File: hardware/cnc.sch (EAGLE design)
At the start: 48 parts, among them IC1 STM32F10XVXT6, Q1 8M, Q2 32K, SW1 SWITCH-SWT-9, SW10 SWITCH-SWT-9, SW11 SWITCH-SWT-9, SW12 SWITCH-SWT-9, SW13 SWITCH-SWT-9, SW14 SWITCH-SWT-9, SW15 SWITCH-SWT-9, SW16 SWITCH-SWT-9, SW2 SWITCH-SWT-9, SW3 SWITCH-SWT-9, SW4 SWITCH-SWT-9, SW5 SWITCH-SWT-9, SW6 SWITCH-SWT-9, SW7 SWITCH-SWT-9, SW8 SWITCH-SWT-9, SW9 SWITCH-SWT-9, U1 LMR14206

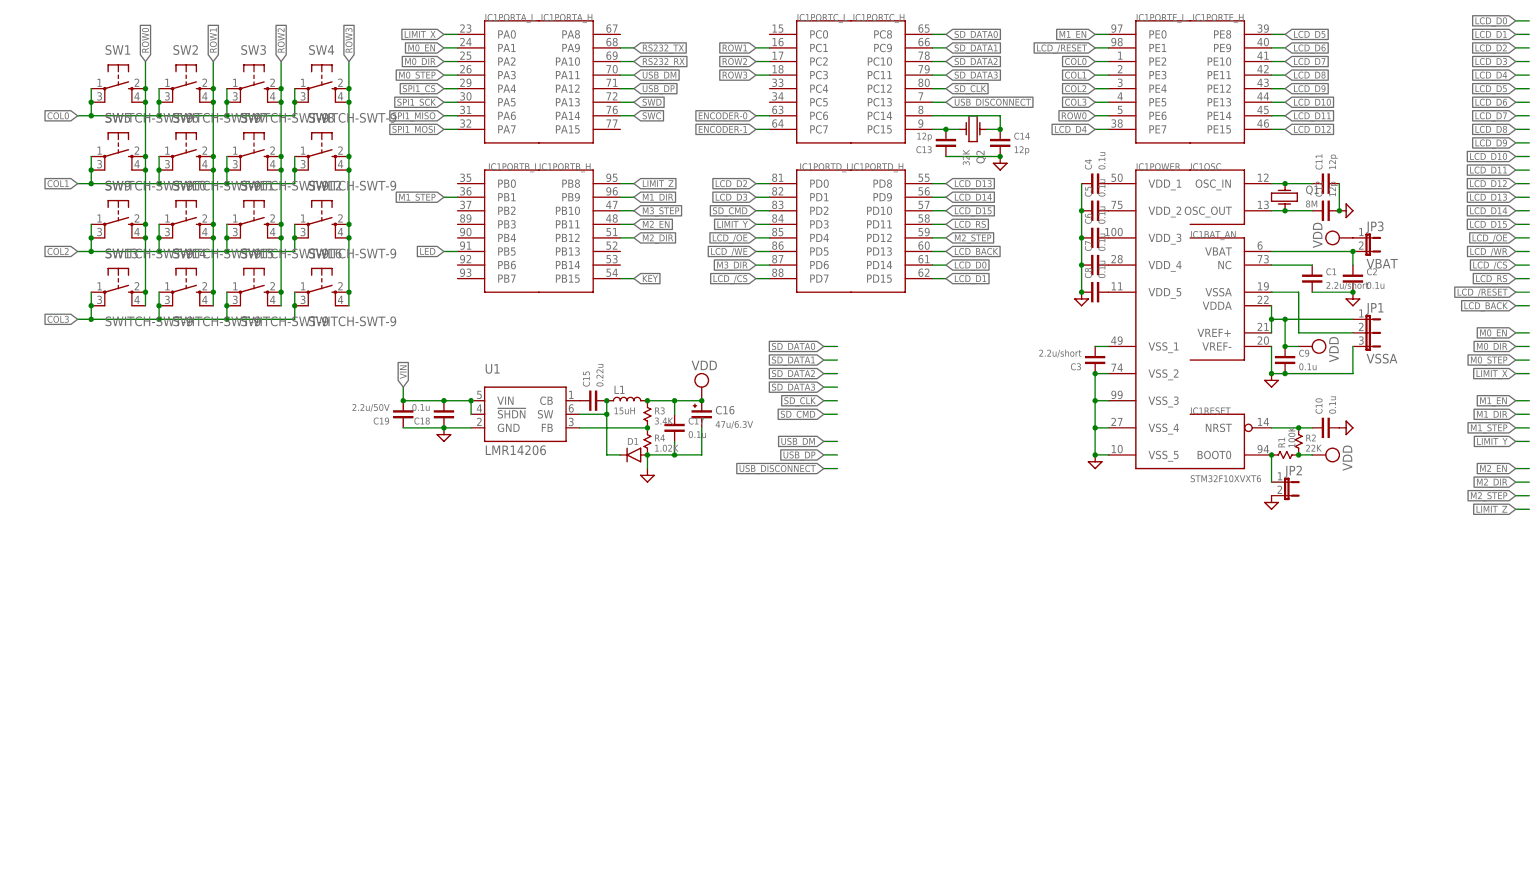
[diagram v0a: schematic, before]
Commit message: Minor changes
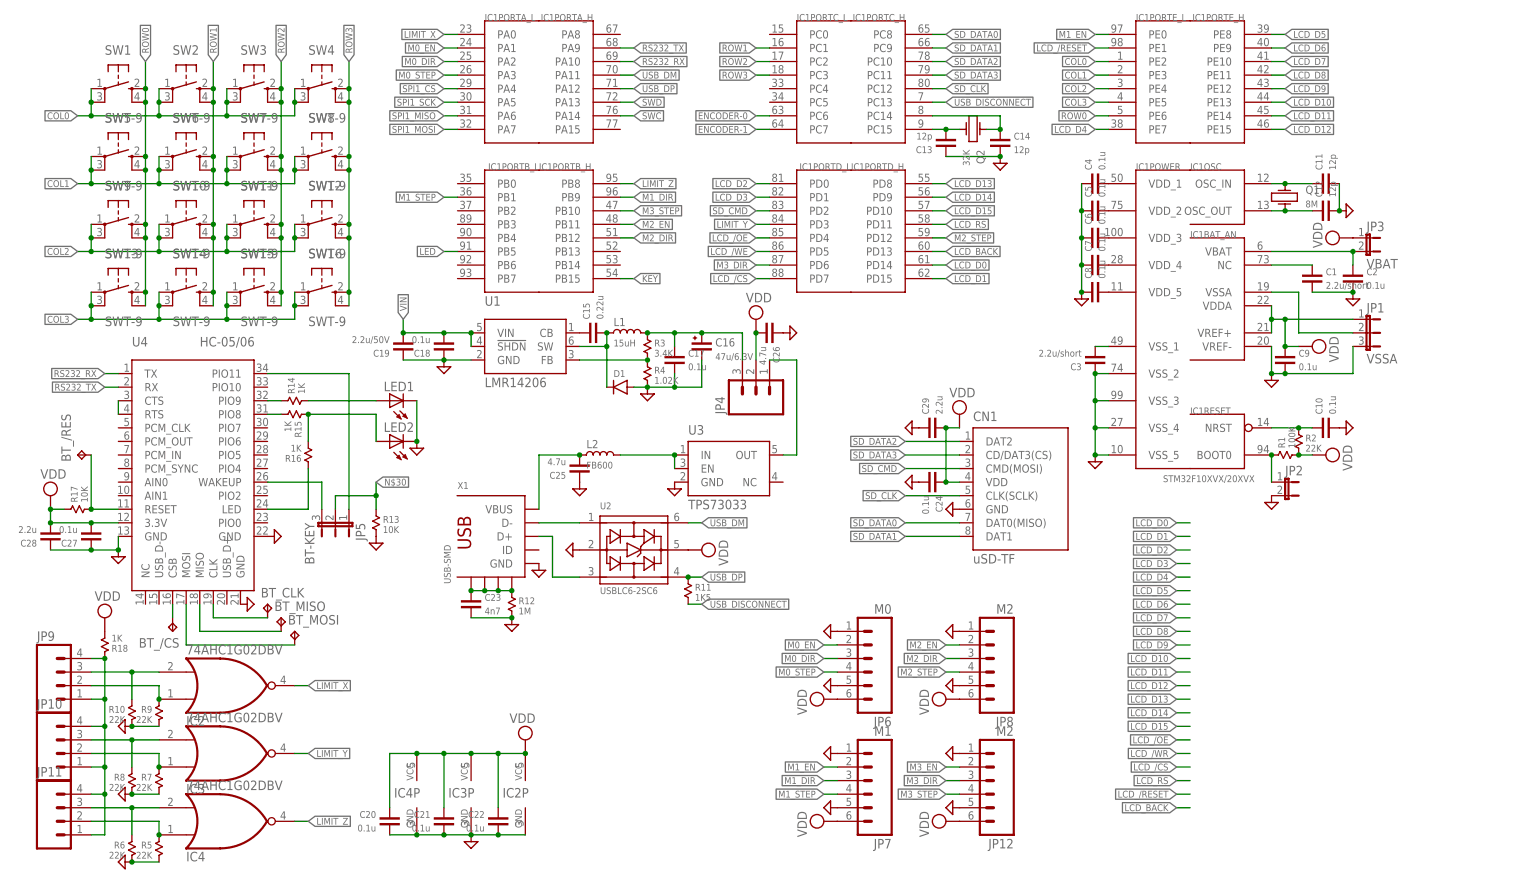
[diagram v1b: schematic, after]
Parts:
- added BT_/CS, BT_/RES, BT_CLK, BT_MISO, BT_MOSI: TPTP12R, testpad:TPTP12R
- added C20, C21, C22, C24, C27: 0.1u, X893:CAP-0603
- added C23: 4n7, X893:CAP-0603
- added C25, C26: 4.7u, X893:CAP-0603
- added C28, C29: 2.2u, X893:CAP-0603
- added CN1: uSD-TF, X893:MICRO-SD-T-FLASH
- added IC2, IC3, IC4: 74AHC1G02DBV, 74xx-little-us:74AHC1G02DBV
- added JP10, JP11, JP9: (no value), SparkFun:M04PTH
- added JP12, JP8: M2, SparkFun:M06SIP
- added JP4: (no value), SparkFun:M03PTH
- added JP5: BT-KEY, SparkFun:JUMPER-3SMD
- added JP6: M0, SparkFun:M06SIP
- added JP7: M1, SparkFun:M06SIP
- added L2: FB600, X893:INDUCTOR-0603
- added LED1, LED2: (no value), led:LEDCHIP-LED0603
- added R10, R5, R6, R7, R8, R9: 22K, X893:RESISTOR-0603
- added R11: 1K5, X893:RESISTOR-0603
- added R12: 1M, X893:RESISTOR-0603
- added R13, R17: 10K, X893:RESISTOR-0603
- added R14, R15, R16, R18: 1K, X893:RESISTOR-0603
- added U2: USBLC6-2SC6, X893:USBLC6-2SC6
- added U3: TPS73033, X893:TPS73033
- added U4: HC-05/06, X893:SEEDI-BT
- added X1: USB-SMD, X893:USB-SMD
- IC1: value STM32F10XVXT6 -> STM32F10XVX/20XVX
- SW1, SW10, SW11, SW12, SW13, SW14, SW15, SW16, SW2, SW3, SW4, SW5, SW6, SW7, SW8, SW9: value SWITCH-SWT-9 -> SWT-9
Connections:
- new net 3V3: C16.+, C17.2, JP4.3, L1.2, R3.1
- new net M3_EN: JP12.2
- new net MAX-X: IC2A.I0, JP9.2, R9.1
- new net MAX-Y: IC3A.I0, JP10.2, R7.1
- new net MAX-Z: IC4A.I0, JP11.2, R5.1
- new net MIN-X: IC2A.I1, JP9.3, R10.1
- new net MIN-Y: IC3A.I1, JP10.3, R8.1
- new net MIN-Z: IC4A.I1, JP11.3, R6.1
- new net N$14: U2.IO1@1, X1.D-
- new net N$20: U2.IO2@1, X1.D+
- new net N$21: U4.CTS, U4.RTS
- new net N$22: C23.2, R12.1, X1.GND@1, X1.GND@2, X1.GND@3, X1.GND@4
- new net N$23: JP4.1, U3.OUT
- new net N$24: L2.2, U3.EN, U3.IN
- new net N$25: JP5.1, U4.PIO11
- new net N$26: R14.1, U4.PIO9
- new net N$27: R15.2, U4.PIO8
- new net N$28: R16.1, U4.LED
- new net N$29: JP5.3, U4.WAKEUP
- new net N$30: JP5.2, R13.1
- new net N$31: LED2.A, R15.1, R16.2
- new net N$32: LED1.A, R14.2
- new net N$33: JP10.1, JP10.4, JP11.1, JP11.4, JP9.1, JP9.4, R18.1
- new net N$34: BT_/CS.TP, U4.CSB
- new net N$35: BT_/RES.TP, R17.2, U4.RESET
- new net N$36: BT_MOSI.TP, U4.MOSI
- new net N$37: BT_MISO.TP, U4.MISO
- new net N$38: BT_CLK.TP, U4.CLK
- new net VUSB: C25.1, L2.1, X1.VBUS
- net GND: now also C20.1, C21.1, C22.1, C23.1, C24.1, C25.2, C26.2, C27.2, C28.2, C29.2, CN1.GND, IC2P.GND, IC3P.GND, IC4P.GND, JP12.1, JP12.5, JP6.1, JP6.5, JP7.1, JP7.5, JP8.1, JP8.5, LED1.C, LED2.C, R10.2, R12.2, R13.2, R5.2, R6.2, R7.2, R8.2, R9.2, U2.GND, U3.GND, U4.GND@1, U4.GND@2, U4.GND@3, X1.GND@0
- net LIMIT_X: now also IC2A.O
- net LIMIT_Y: now also IC3A.O
- net LIMIT_Z: now also IC4A.O
- net M0_DIR: now also JP6.3
- net M0_EN: now also JP6.2
- net M0_STEP: now also JP6.4
- net M1_DIR: now also JP7.3
- net M1_EN: now also JP7.2
- net M1_STEP: now also JP7.4
- net M2_DIR: now also JP8.3
- net M2_EN: now also JP8.2
- net M2_STEP: now also JP8.4
- net M3_DIR: now also JP12.3
- net M3_STEP: now also JP12.4
- net RS232_RX: now also U4.TX
- net RS232_TX: now also U4.RX
- net USB_DISCONNECT: now also R11.2
- net USB_DM: now also U2.IO1@2
- net USB_DP: now also R11.1, U2.IO2@2
- net VDD: now also C20.2, C21.2, C22.2, C24.2, C26.1, C27.1, C28.1, C29.1, CN1.VDD, IC2P.VCC, IC3P.VCC, IC4P.VCC, JP12.6, JP4.2, JP6.6, JP7.6, JP8.6, R17.1, R18.2, U2.VBUS, U4.3.3V; no longer C16.+, C17.2, L1.2, R3.1
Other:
- moved on the sheet: C15, C16, C17, C18, C19, D1, L1, R3, R4, U1
